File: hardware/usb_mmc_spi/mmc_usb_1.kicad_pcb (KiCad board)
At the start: 2 copper layers, 47.6 x 27.3 mm, 27 parts, among them J351 MINI-USB-5P-3400020P1, K351 CONN_3, M351 CONN_1, M352 CONN_1, P351 CONN_5X2, P352 MICRO-SDCARD-CONNECTOR-330006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, P353 CONN_10X2, P354 CONN_10X2, P355 CONN_1, P356 CONN_1, U351 FT232RL

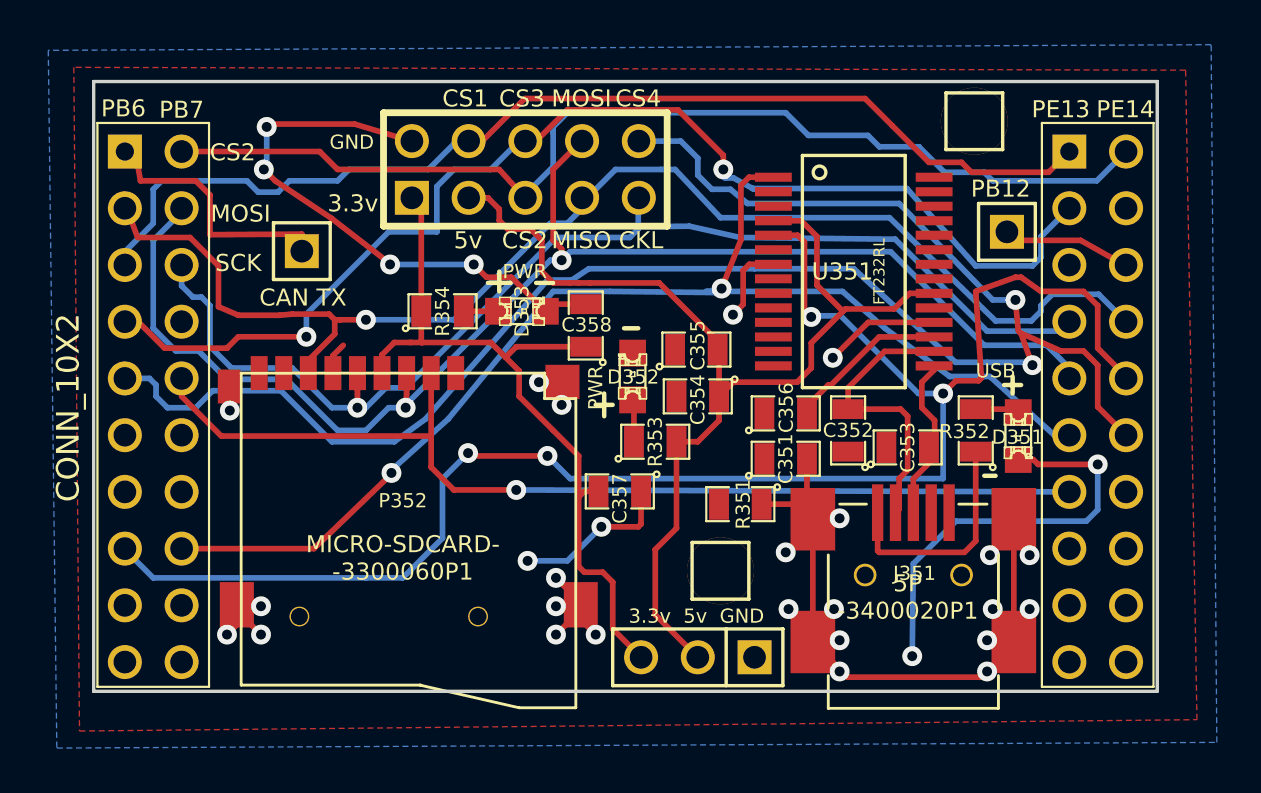
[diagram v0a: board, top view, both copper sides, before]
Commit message: update pcb files
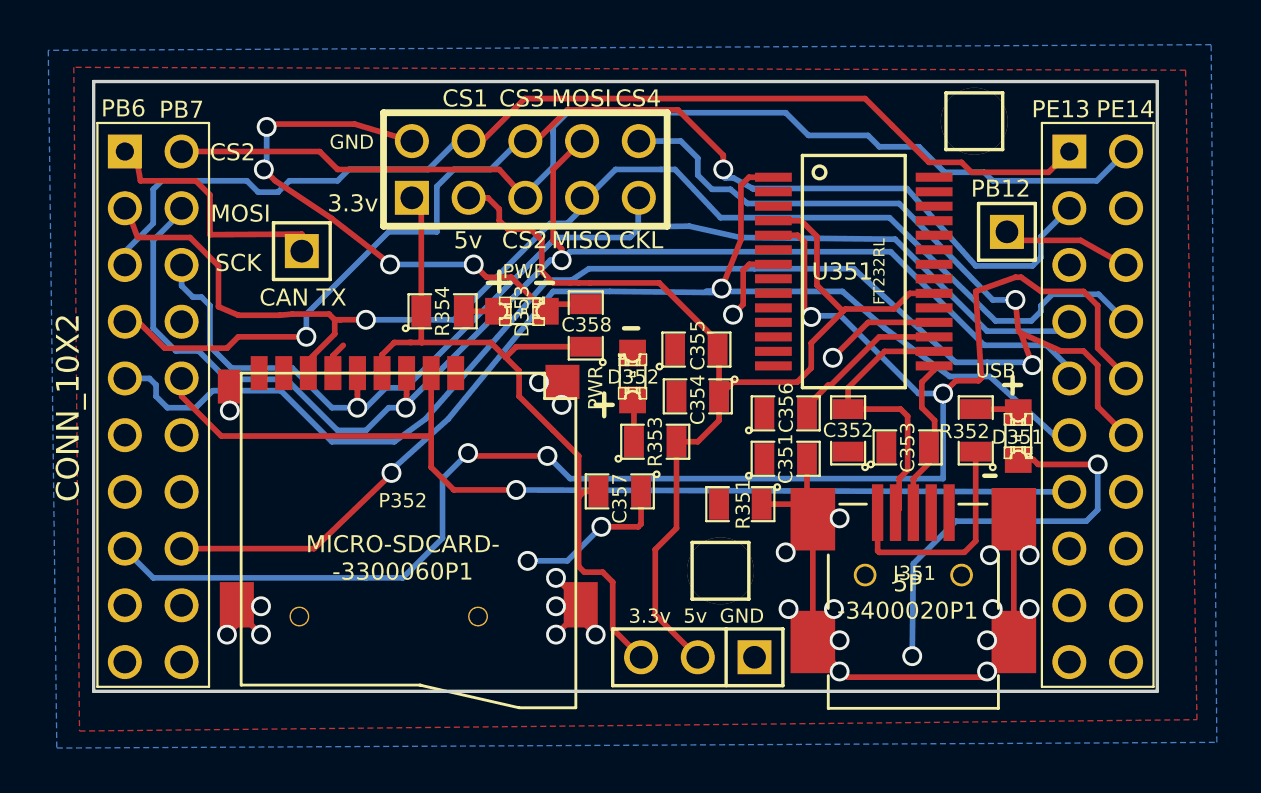
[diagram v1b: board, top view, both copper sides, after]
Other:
- net class Default removed
